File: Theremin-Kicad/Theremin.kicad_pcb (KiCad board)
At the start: 2 copper layers, 131.8 x 80 mm, 36 parts, among them CON1 BARREL_JACK, P1 SENSOR_1_NOTA, P2 SENSOR_2_VOL, P3 FPGA_OUTS, P4 FPGA_INS, P5 AUDIO_OUT, P6 CONN_2, SW1 VOL_UP, SW2 VOL_DOWN, SW3 PITCH_UP, SW4 PITCH_DOWN, SW5 MODE, SW6 SET, U1 NCP1117ST33T3G, U2 LM78M05CT, U3 X9C104P

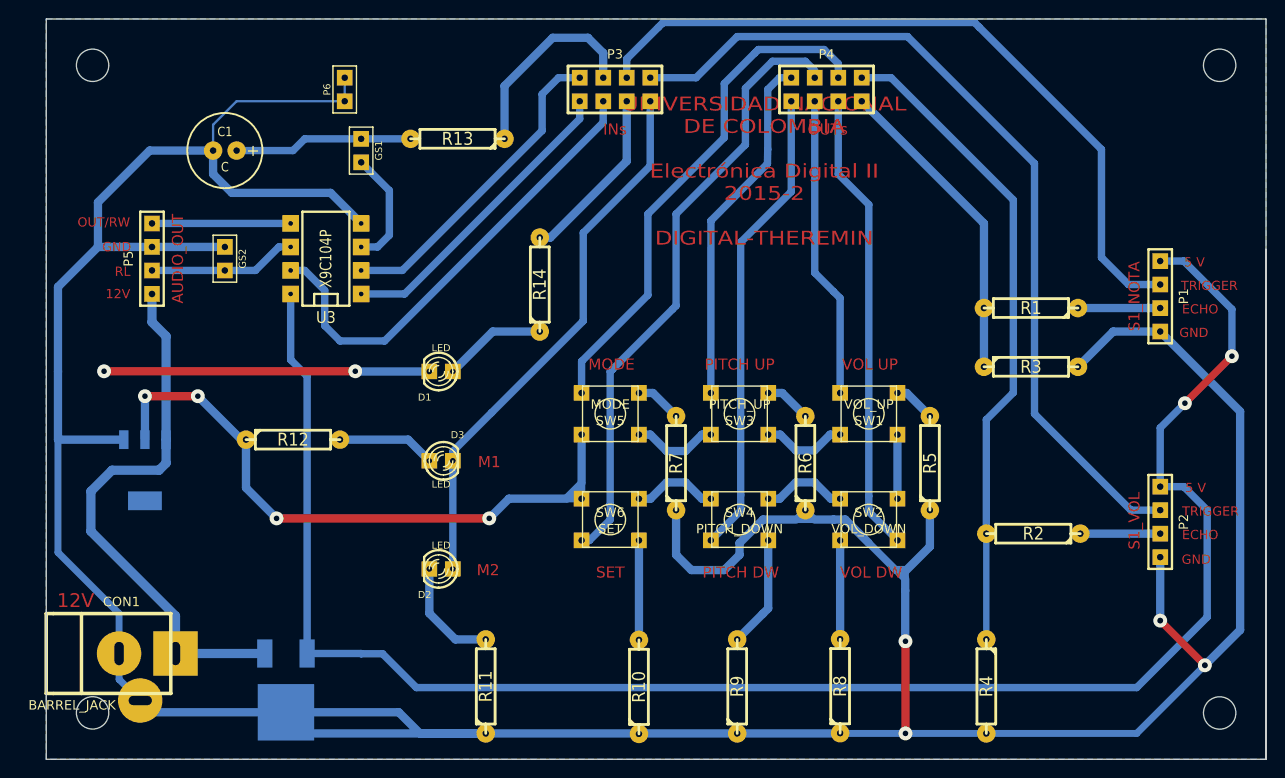
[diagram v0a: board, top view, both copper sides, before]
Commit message: Revert "25Nov"
This reverts commit 00753210b0956ffd3ebe100875fb0ab7c5a08096.
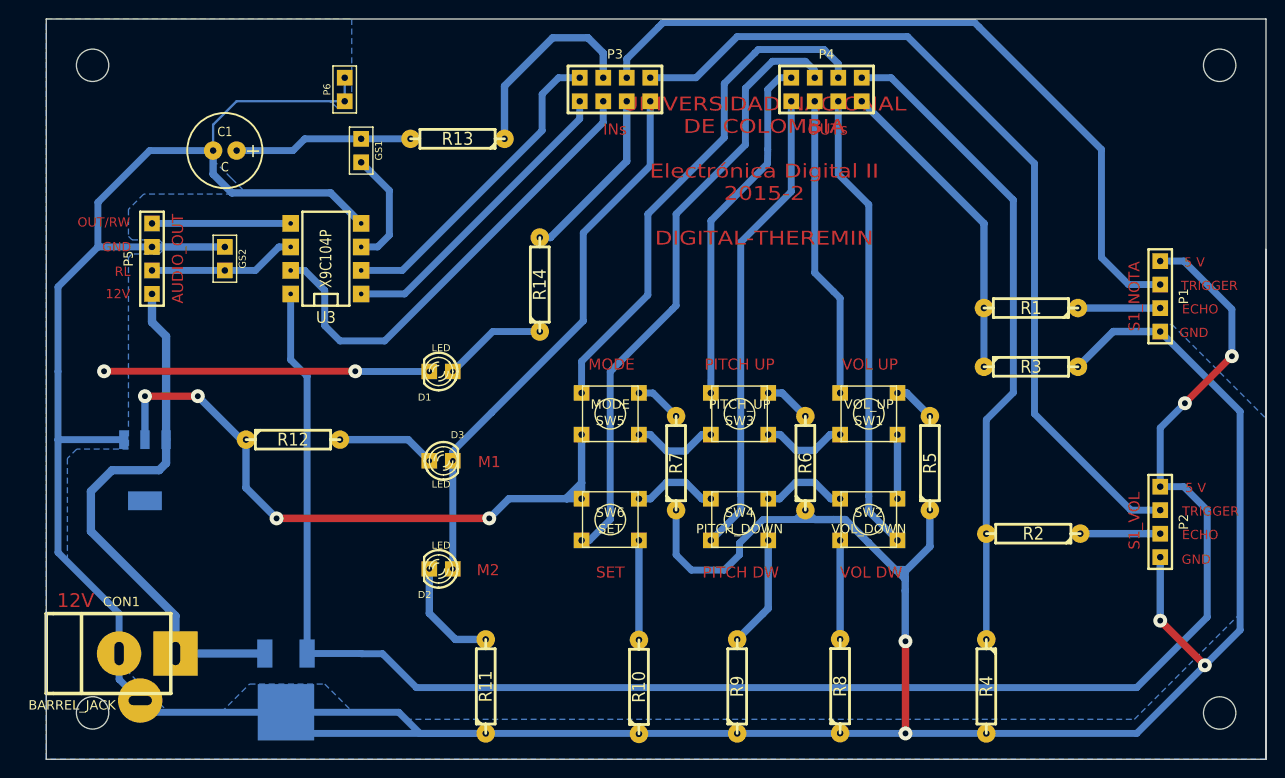
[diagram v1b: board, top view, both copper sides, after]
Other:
- net class 1 added: clearance 0.254, trace_width 0.3, via_dia 0.889, via_drill 0.635
- net class 2 added: clearance 0.254, trace_width 0.35, via_dia 0.889, via_drill 0.635
- net class 3 added: clearance 0.254, trace_width 0.4, via_dia 0.889, via_drill 0.635
- net class 4 added: clearance 0.254, trace_width 0.45, via_dia 0.889, via_drill 0.635
- net class 5 added: clearance 0.254, trace_width 0.5, via_dia 0.889, via_drill 0.635
- net class 6 added: clearance 0.254, trace_width 0.65, via_dia 1.5, via_drill 0.6
- net class nwo removed

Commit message: 25Nov
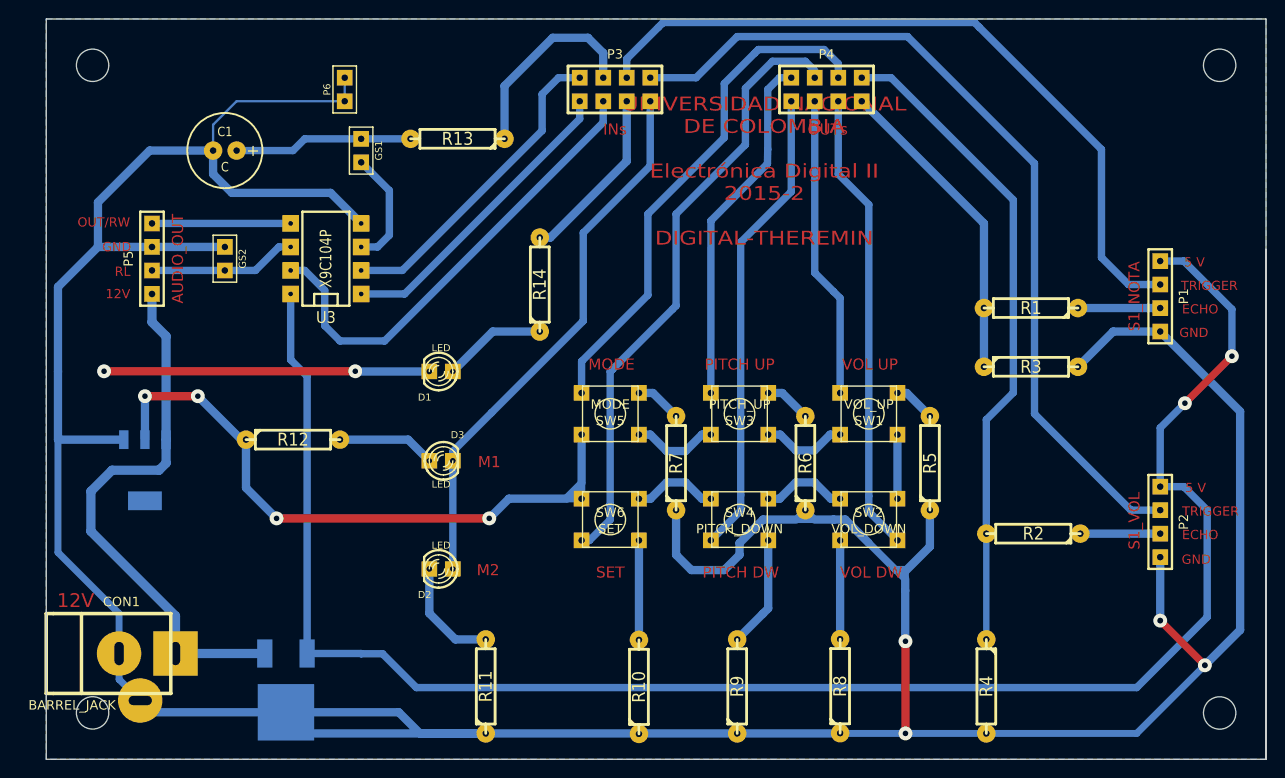
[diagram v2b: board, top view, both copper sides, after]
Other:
- net class 1 removed
- net class 2 removed
- net class 3 removed
- net class 4 removed
- net class 5 removed
- net class 6 removed
- net class nwo added: clearance 0.254, trace_width 1, via_dia 1.5, via_drill 0.6
